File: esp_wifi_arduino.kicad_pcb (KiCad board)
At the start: 2 copper layers, 30 x 50 mm, 30 parts, among them CON1 AVR-ISP-6, IC1 ATMEGA328P-A, P1 CONN_15, P2 CONN_15, SW1 SW_PUSH, SW2 SW_PUSH, SW3 DIPSW4, U1 ADG3304, U2 ESP-WROOM-02, U3 NJM2391DL1-33, X1 16MHz

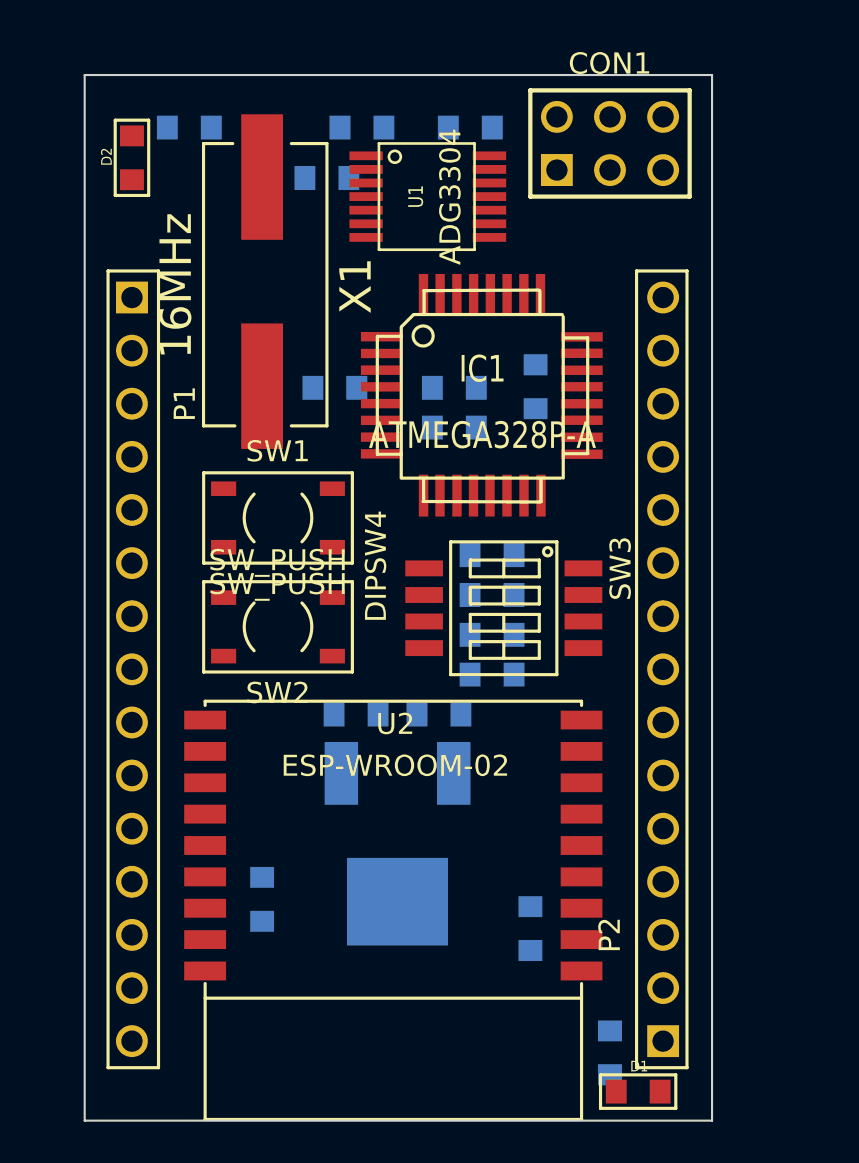
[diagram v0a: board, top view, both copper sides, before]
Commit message: Circuit Create
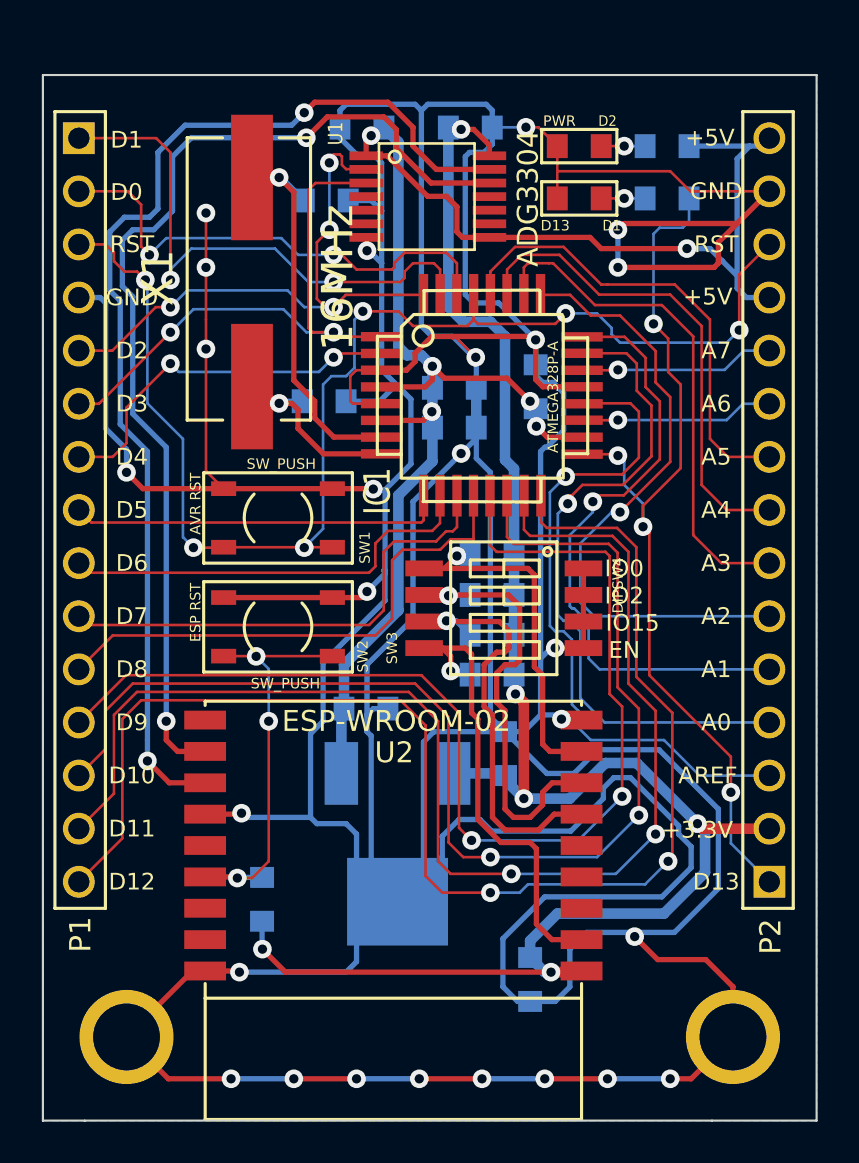
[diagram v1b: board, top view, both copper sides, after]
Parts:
- removed CON1: AVR-ISP-6, pin_array_3x2
- added P3: CONN_1, M3_Drill, F.Cu at (77.0, 76.0)
- added P4: CONN_1, M3_Drill, F.Cu at (48.0, 76.0)
- moved D1 42.8 mm to (69.7, 35.9)
- moved R1 40.9 mm to (73.9, 35.9), turned to 180 degrees
- moved R2 22.9 mm to (73.9, 33.4)
- moved D2 21.4 mm to (69.7, 33.4), turned to 180 degrees
- moved C4 10.7 mm to (57.4, 45.6)
- moved P2 9.16 mm to (78.7, 63.5)
- moved C5 8.97 mm to (57.5, 36.0)
- moved P1 8.03 mm to (45.7, 38.1)
- moved C9 3.65 mm to (66.1, 62.5), turned to 90 degrees
- moved C10 2.33 mm to (67.3, 73.2), turned to 270 degrees
- moved C8 0.55 mm to (59.4, 60.3)
- moved X1 0.48 mm to (54.0, 39.9), turned to 90 degrees
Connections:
- U1 pad 12: /ArduinoRX33 -> /ArduinoTX33
- U1 pad 13: /ArduinoTX33 -> /ArduinoRX33
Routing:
- net GND: track 0.00 -> 393.0 mm, vias 0 -> 26
- net +3.3V: track 0.00 -> 86.1 mm, vias 0 -> 6
- net +5V: track 0.00 -> 84.4 mm, vias 0 -> 6
- net /D12: track 0.00 -> 65.9 mm, vias 0 -> 2
- net /RESET: track 0.00 -> 63.0 mm, vias 0 -> 6
- net /D11: track 0.00 -> 61.9 mm, vias 0 -> 2
- net /D10: track 0.00 -> 58.0 mm, vias 0 -> 2
- net /D9: track 0.00 -> 54.3 mm, vias 0 -> 2
- net /ArduinoRX33: track 0.00 -> 53.4 mm, vias 0 -> 2
- net /ArduinoTX33: track 0.00 -> 50.2 mm, vias 0 -> 2
- net /D13: track 0.00 -> 43.5 mm, vias 0 -> 4
- net /A0: track 0.00 -> 32.4 mm, vias 0 -> 1
- net /AREF: track 0.00 -> 32.2 mm, vias 0 -> 1
- net /A2: track 0.00 -> 30.3 mm, vias 0 -> 1
- net /A1: track 0.00 -> 29.9 mm, vias 0 -> 1
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- added copper zone on B.Cu, net GND
- added copper zone on F.Cu, net GND
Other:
- board size 30 x 50 mm -> 37 x 50 mm
- rule trace_min: 0.254 -> 0.127
- board text added: "+3.3V"
- board text added: "+5V"
- board text added: "A0"
- board text added: "A1"
- board text added: "A2"
- board text added: "A3"
- board text added: "A4"
- board text added: "A5"
- board text added: "A6"
- board text added: "A7"
- board text added: "AREF"
- board text added: "AVR RST"
- board text added: "Asumono-001-Rev.A"
- board text added: "Asumonoduino-Wifi"
- board text added: "D0"
- board text added: "D1"
- board text added: "D10"
- board text added: "D11"
- board text added: "D12"
- board text added: "D13"
- board text added: "D2"
- board text added: "D3"
- board text added: "D4"
- board text added: "D5"
- board text added: "D6"
- board text added: "D7"
- board text added: "D8"
- board text added: "D9"
- board text added: "EN"
- board text added: "ESP RST"
- board text added: "GND"
- board text added: "IO0"
- board text added: "IO15"
- board text added: "IO2"
- board text added: "PWR"
- board text added: "RST"
